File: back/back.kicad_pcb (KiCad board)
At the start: 2 copper layers, 65 x 70 mm, 20 parts, among them J1 Screw_Terminal_01x02, J2 Screw_Terminal_01x02, J3 Screw_Terminal_01x02, Q1 IRF510, U1 NE555

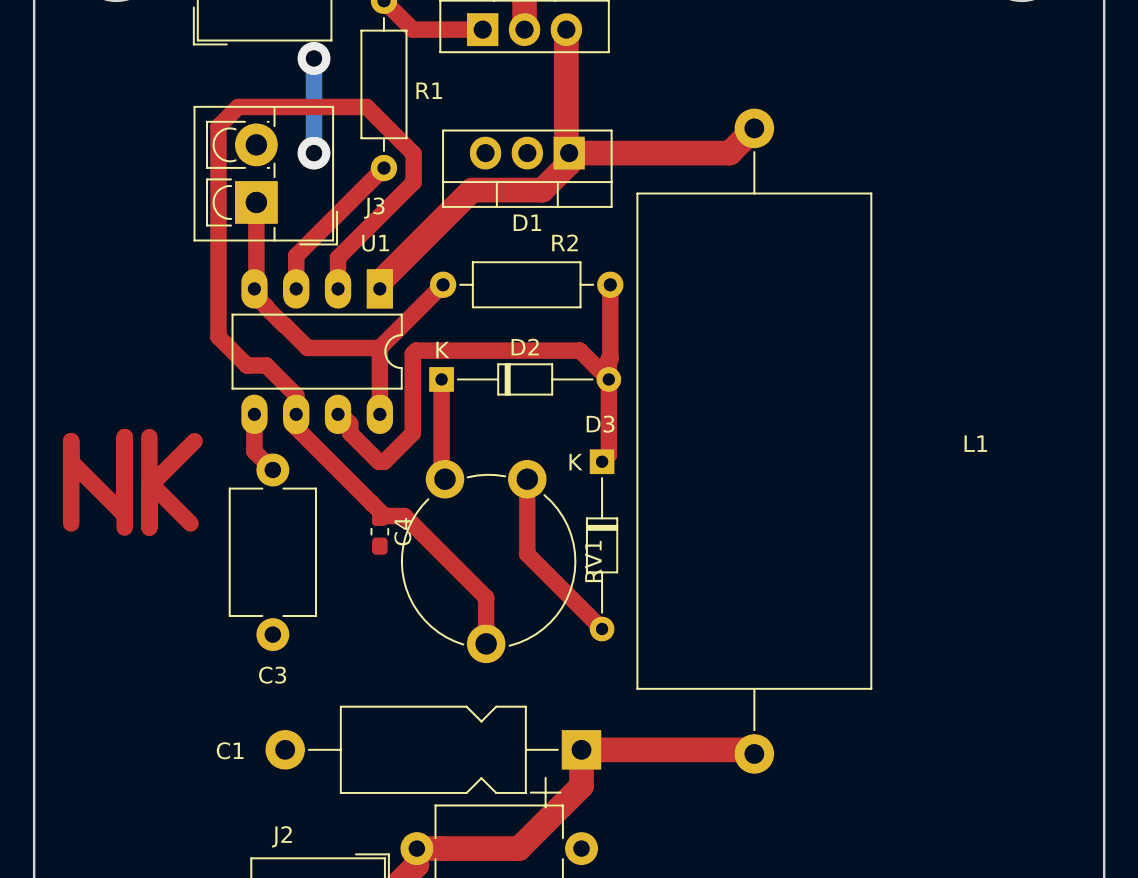
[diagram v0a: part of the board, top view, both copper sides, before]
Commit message: wersja nie dzialajaca
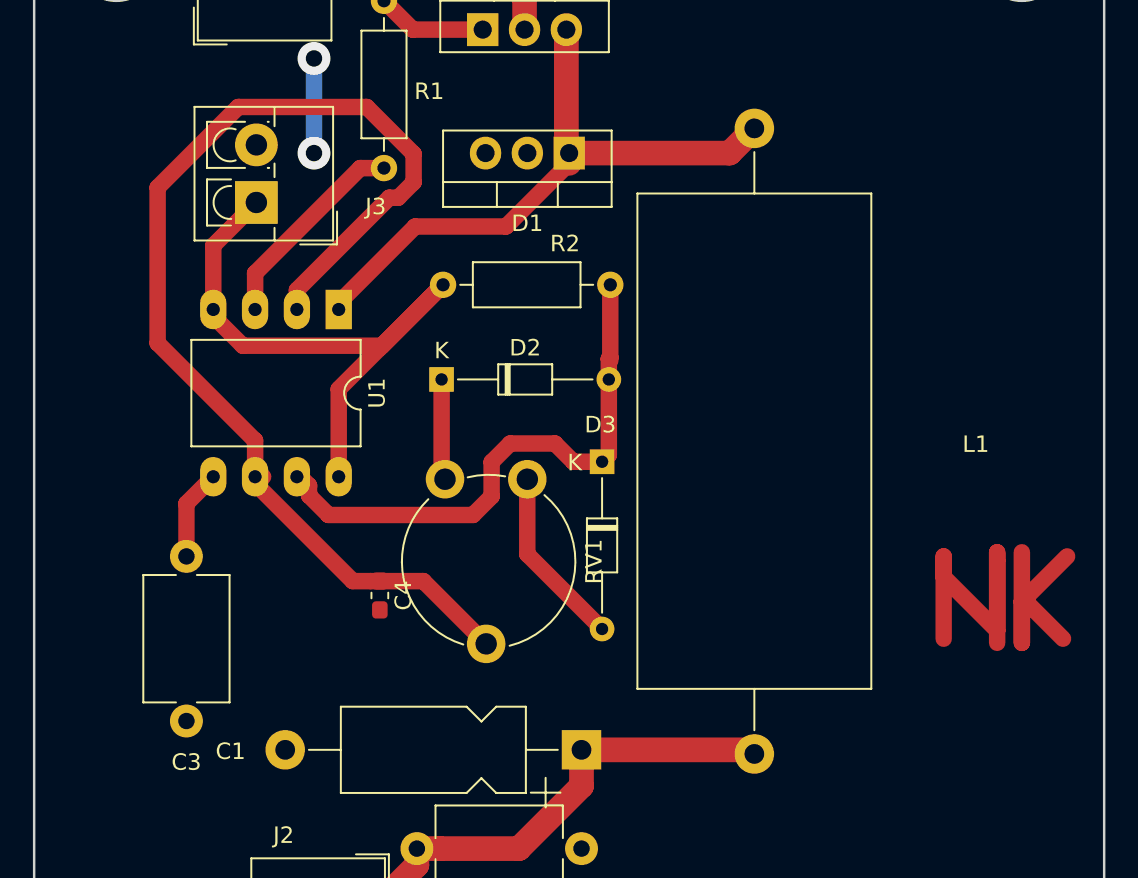
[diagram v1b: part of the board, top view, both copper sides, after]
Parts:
- U1: footprint Package_DIP:DIP-8_W7.62mm_LongPads -> Package_DIP:DIP-8_W10.16mm_LongPads
- moved C3 7.42 mm to (146.8, 83.8)
- moved C4 3.88 mm to (158.5, 86.1)
- moved U1 2.80 mm to (156.0, 68.8)
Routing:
- net /RST: track 24.1 -> 43.9 mm
- net Net-(C3-Pad1): track 3.84 -> 20.8 mm
- net (no net): track 36.4 -> 21.1 mm
- net /TRIG: track 64.0 -> 70.5 mm
- net /GNDCLK: track 35.1 -> 38.1 mm
- net /Q_Base: track 9.95 -> 12.7 mm
- net Net-(D2-Pad2): track 35.8 -> 34.4 mm

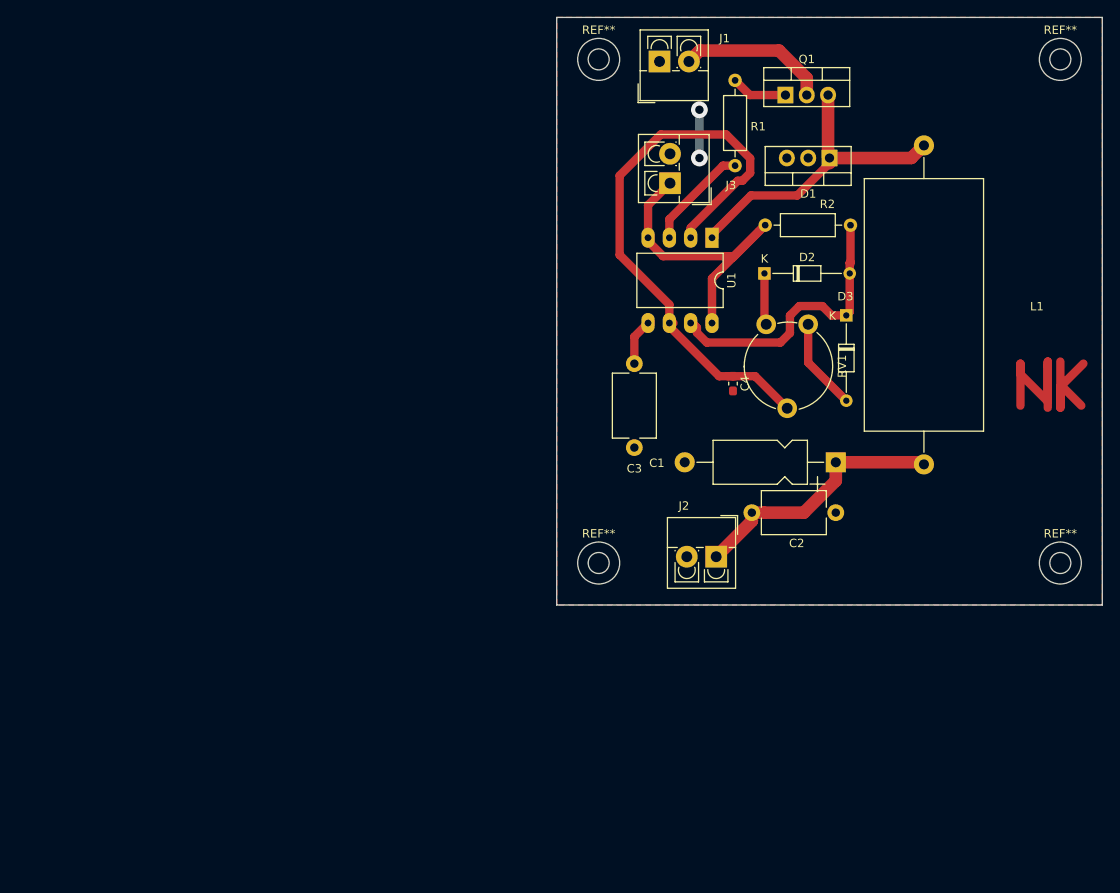
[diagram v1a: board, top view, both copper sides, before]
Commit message: final 6.10
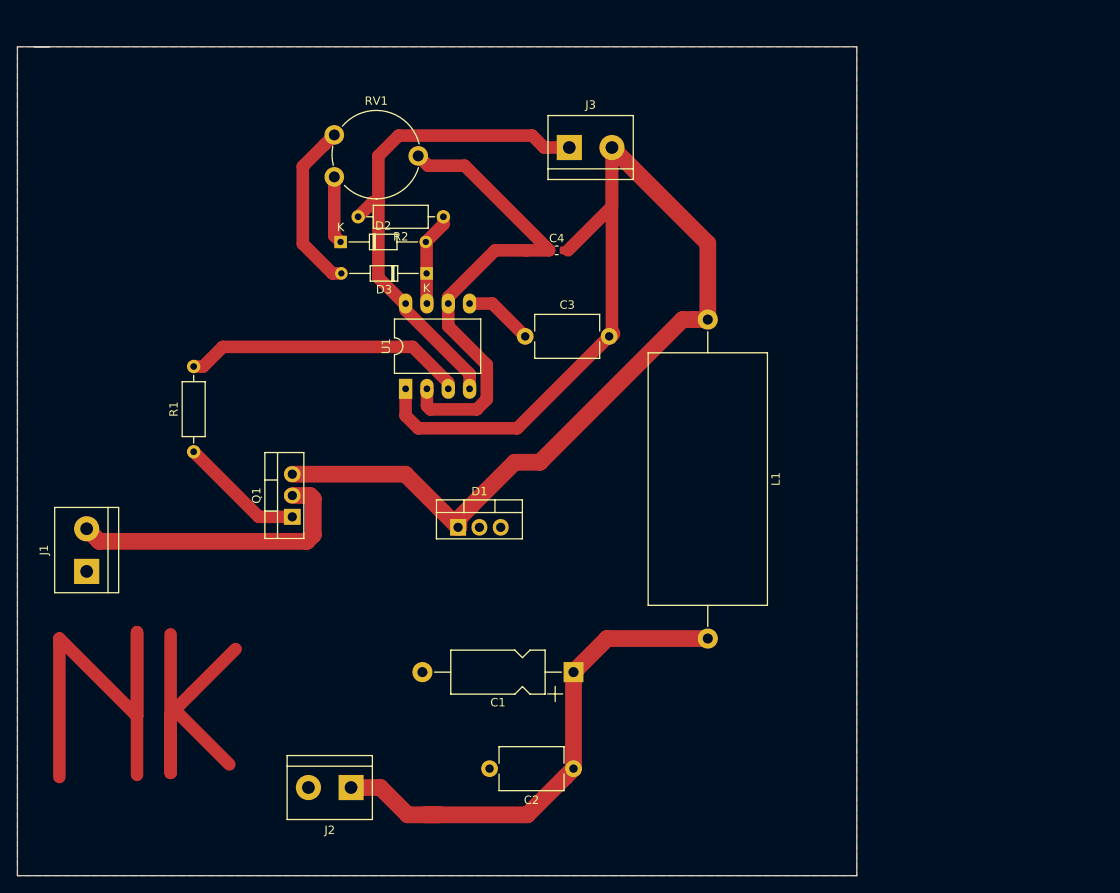
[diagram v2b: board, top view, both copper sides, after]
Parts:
- removed REF** (x4): MountingHole_2.5mm, MountingHole:MountingHole_2.5mm
- C1: value 1u -> 22u
- J1, J2, J3: footprint TerminalBlock_4Ucon:TerminalBlock_4Ucon_1x02_P3.50mm_Vertical -> TerminalBlock:TerminalBlock_bornier-2_P5.08mm
- L1: footprint back:ind_W60mm_D19mm_P38mm -> Footprints:ind_W60mm_D19mm_P38mm
- moved J1 91.4 mm to (81.5, 108.5), turned to 90 degrees
- moved R1 78.2 mm to (94.2, 94.2), turned to 90 degrees
- moved Q1 77.3 mm to (106.0, 102.0), turned to 90 degrees
- moved D1 62.4 mm to (125.8, 103.2), turned to 0 degrees
- moved RV1 54.4 mm to (111.0, 61.5), turned to 0 degrees
- moved J2 51.5 mm to (113.0, 134.2)
- moved D2 50.6 mm to (111.8, 69.2)
- moved D3 50.2 mm to (122.0, 73.0), turned to 180 degrees
- moved R2 48.5 mm to (124.0, 66.2)
- moved U1 40.7 mm to (119.5, 86.8), turned to 90 degrees
- moved C1 40.0 mm to (139.5, 120.5)
- moved C2 37.2 mm to (139.5, 132.0), turned to 180 degrees
- moved L1 33.1 mm to (155.5, 78.5)
- moved C4 26.3 mm to (137.5, 70.2), turned to 0 degrees
- moved C3 13.4 mm to (133.8, 80.5), turned to 0 degrees
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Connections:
- C3 pad 2: GND -> /GNDCLK
- C4 pad 2: GND -> /GNDCLK
- J3 pad 2: GND -> /GNDCLK
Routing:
- net /GNDCLK: track 38.1 -> 157.9 mm
- net (no net): track 21.1 -> 100.4 mm
- net Net-(C1-Pad1): track 31.8 -> 61.0 mm
- net Net-(D2-Pad2): track 34.4 -> 11.3 mm
- net /Q_Base: track 12.7 -> 33.8 mm
- net Net-(J1-Pad2): track 17.9 -> 34.9 mm
- net /RST: track 43.9 -> 59.8 mm
- net Net-(C3-Pad1): track 20.8 -> 8.25 mm
- net /TRIG: track 70.5 -> 58.5 mm
- net Net-(D3-Pad2): track 11.0 -> 20.6 mm
- net Net-(Q1-Pad1): track 6.72 -> 15.0 mm
- net GND: track 5.75 -> 0.00 mm, vias 2 -> 0
- net Net-(D2-Pad1): track 6.15 -> 8.06 mm
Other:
- board size 65 x 70 mm -> 100 x 98.8 mm
- net class Default: trace_width 1 -> 1.5; via_dia 0.8 -> 1; via_drill 0.4 -> 0.5
- net class Power: trace_width 1.5 -> 2; via_dia 0.8 -> 1.5; via_drill 0.4 -> 0.5
